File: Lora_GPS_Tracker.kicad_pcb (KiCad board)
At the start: 4 copper layers, 52.4 x 30.8 mm, 43 parts, among them J101 USB_C_Receptacle_USB2.0_16P, J102 Conn_01x02, J103 Conn_01x05_Pin, J104 Conn_01x02, J105 Conn_01x02, J106 Conn_Coaxial, J107 Conn_Coaxial, U101 STM32G031G6Ux, U102 MCP73831-2-OT, U103 TPS631000DRLR, U104 GP-02, U105 E220-900T22S

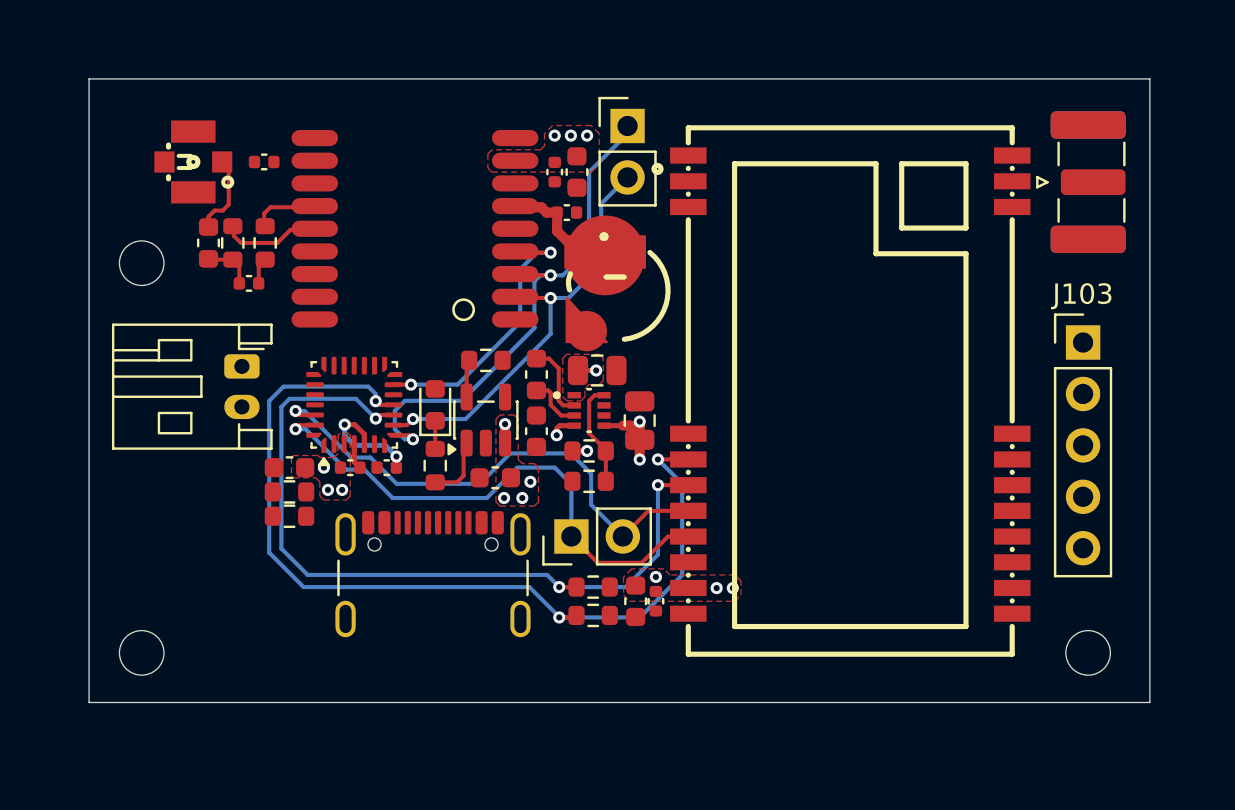
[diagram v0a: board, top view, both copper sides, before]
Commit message: feat: finish baisc layout
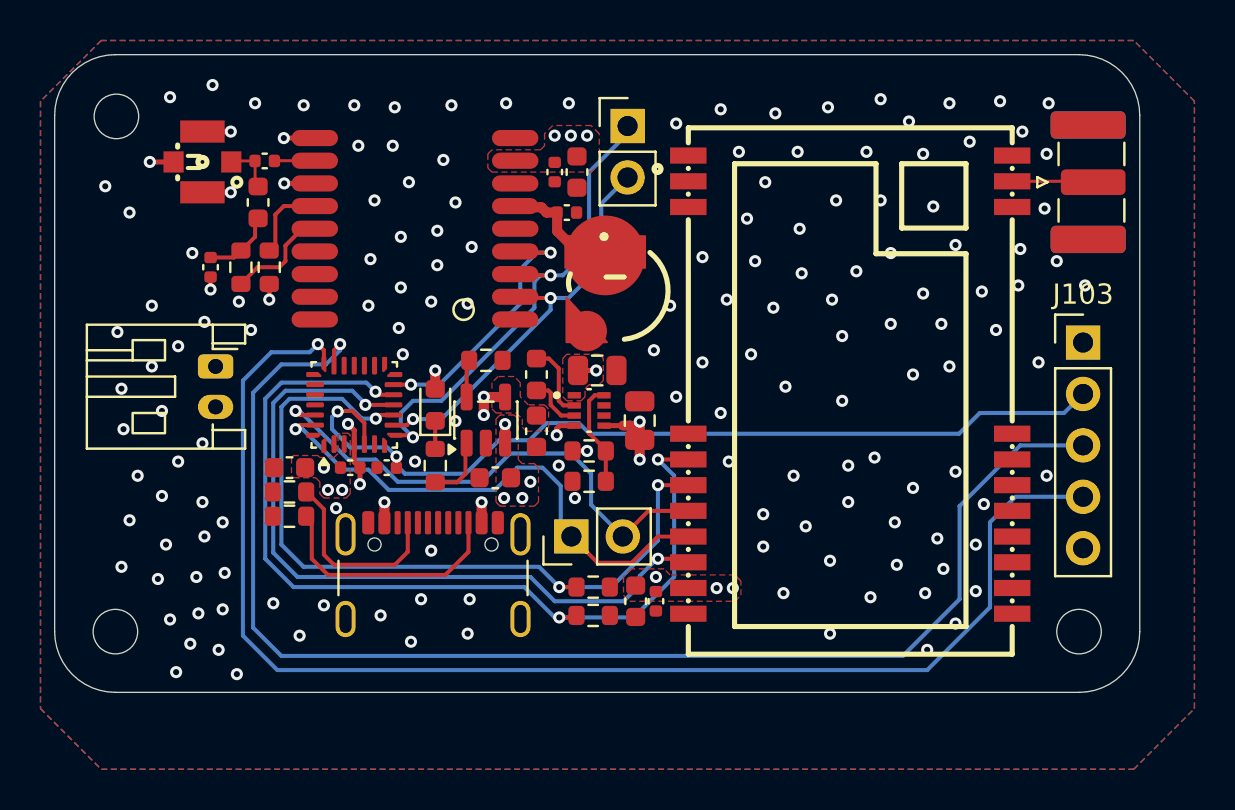
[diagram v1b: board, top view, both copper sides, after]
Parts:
- moved H101 7.36 mm to (41.8, 86.8)
- moved L102 3.16 mm to (48.8, 91.0)
- moved C115 2.06 mm to (46.4, 94.2), turned to -90 degrees
- moved H102 1.67 mm to (41.7, 112.2)
- moved J102 1.30 mm to (46.6, 99.1)
- moved R110 1.26 mm to (47.9, 94.2), turned to 90 degrees
- moved R107 1.22 mm to (49.3, 94.2)
- moved R101 1.20 mm to (50.3, 106.5)
- moved R102 1.20 mm to (50.3, 105.3)
- moved H103 1.14 mm to (89.3, 112.2)
- moved J107 0.45 mm to (46.0, 89.0)
- moved C114 0.06 mm to (49.1, 89.0)
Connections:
- J103 pad 3: /SWCLK -> /SWDIO
- J103 pad 4: /SWDIO -> /SWCLK
- U101 pad 11: /M0 -> /AUX
- U101 pad 12: /AUX -> /M0
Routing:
- net /SWDIO: track 0.00 -> 66.8 mm, vias 0 -> 1
- net /SWCLK: track 0.00 -> 66.4 mm, vias 0 -> 1
- net /NRST: track 5.74 -> 43.9 mm
- net /AUX: track 0.00 -> 36.6 mm, vias 0 -> 2
- net +BATT: track 23.7 -> 6.42 mm
- net Net-(J101-CC2): track 0.00 -> 12.2 mm
- net Net-(J101-CC1): track 0.00 -> 9.53 mm
- net GND: track 2.59 -> 11.9 mm, vias 0 -> 160
- net VBUS: track 0.00 -> 4.89 mm, vias 0 -> 5
- net Net-(J106-In): track 0.00 -> 4.02 mm
- net Net-(U104-RF_IN): track 0.00 -> 2.00 mm
- net Net-(J107-In): track 4.00 -> 2.46 mm
- net /GPS_TX: track 25.9 -> 24.4 mm
- net Net-(C115-Pad1): track 2.52 -> 3.53 mm
- net Net-(U104-IO8): track 3.25 -> 4.02 mm
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- added copper zone on B.Cu, net GND
- added copper zone on F.Cu, net GND
- added copper zone on In1.Cu, net GND
- added copper zone on F.Cu, net VBUS
- added copper zone on In2.Cu, net VBUS
- removed copper zone on In1.Cu, net (none)
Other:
- board size 52.4 x 30.8 mm -> 53.6 x 31.5 mm
